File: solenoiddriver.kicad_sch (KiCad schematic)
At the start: 14 parts, among them Q501 WSP6946, Q502 WSP6946

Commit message: Assign footprints
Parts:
- D501, D502, D503, D504: footprint (none) -> Diode_SMD:D_SMA_Handsoldering
- R501, R502, R503, R504, R505, R506, R507, R508: footprint (none) -> Resistor_SMD:R_0805_2012Metric_Pad1.20x1.40mm_HandSolder
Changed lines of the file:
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@@
     (property "Reference" "R501" (id 0) (at 64.77 44.45 90))
     (property "Value" "150R" (id 1) (at 64.77 46.99 90))
-    (property "Footprint" "" (id 2) (at 64.77 48.768 90)
+    (property "Footprint" "Resistor_SMD:R_0805_2012Metric_Pad1.20x1.40mm_HandSolder" (id 2) (at 64.77 48.768 90)
       (effects (font (size 1.27 1.27)) hide)
     )
@@
     (property "Reference" "R502" (id 0) (at 64.77 76.2 90))
     (property "Value" "150R" (id 1) (at 64.77 78.74 90))
-    (property "Footprint" "" (id 2) (at 64.77 76.962 90)
+    (property "Footprint" "Resistor_SMD:R_0805_2012Metric_Pad1.20x1.40mm_HandSolder" (id 2) (at 64.77 76.962 90)
       (effects (font (size 1.27 1.27)) hide)
     )
@@
       (effects (font (size 1.27 1.27)) (justify left))
     )
-    (property "Footprint" "" (id 2) (at 69.342 52.07 90)
+    (property "Footprint" "Resistor_SMD:R_0805_2012Metric_Pad1.20x1.40mm_HandSolder" (id 2) (at 69.342 52.07 90)
       (effects (font (size 1.27 1.27)) hide)
     )
@@
       (effects (font (size 1.27 1.27)) (justify right))
     )
-    (property "Footprint" "" (id 2) (at 72.898 83.82 90)
+    (property "Footprint" "Resistor_SMD:R_0805_2012Metric_Pad1.20x1.40mm_HandSolder" (id 2) (at 72.898 83.82 90)
       (effects (font (size 1.27 1.27)) hide)
     )
@@
     (property "Reference" "R505" (id 0) (at 149.86 44.45 90))
     (property "Value" "150R" (id 1) (at 149.86 46.99 90))
-    (property "Footprint" "" (id 2) (at 149.86 48.768 90)
+    (property "Footprint" "Resistor_SMD:R_0805_2012Metric_Pad1.20x1.40mm_HandSolder" (id 2) (at 149.86 48.768 90)
       (effects (font (size 1.27 1.27)) hide)
     )
@@
     (property "Reference" "R506" (id 0) (at 149.86 76.2 90))
     (property "Value" "150R" (id 1) (at 149.86 78.74 90))
-    (property "Footprint" "" (id 2) (at 149.86 80.518 90)
+    (property "Footprint" "Resistor_SMD:R_0805_2012Metric_Pad1.20x1.40mm_HandSolder" (id 2) (at 149.86 80.518 90)
       (effects (font (size 1.27 1.27)) hide)
     )
@@
       (effects (font (size 1.27 1.27)) (justify left))
     )
-    (property "Footprint" "" (id 2) (at 154.432 52.07 90)
+    (property "Footprint" "Resistor_SMD:R_0805_2012Metric_Pad1.20x1.40mm_HandSolder" (id 2) (at 154.432 52.07 90)
       (effects (font (size 1.27 1.27)) hide)
     )
@@
       (effects (font (size 1.27 1.27)) (justify left))
     )
-    (property "Footprint" "" (id 2) (at 154.432 83.82 90)
+    (property "Footprint" "Resistor_SMD:R_0805_2012Metric_Pad1.20x1.40mm_HandSolder" (id 2) (at 154.432 83.82 90)
       (effects (font (size 1.27 1.27)) hide)
     )
@@
       (effects (font (size 1.27 1.27)) (justify left))
     )
-    (property "Footprint" "" (id 2) (at 100.33 33.02 0)
+    (property "Footprint" "Diode_SMD:D_SMA_Handsoldering" (id 2) (at 100.33 33.02 0)
       (effects (font (size 1.27 1.27)) hide)
     )
@@
       (effects (font (size 1.27 1.27)) (justify left))
     )
-    (property "Footprint" "" (id 2) (at 100.33 64.77 0)
+    (property "Footprint" "Diode_SMD:D_SMA_Handsoldering" (id 2) (at 100.33 64.77 0)
       (effects (font (size 1.27 1.27)) hide)
     )
@@
       (effects (font (size 1.27 1.27)) (justify left))
     )
-    (property "Footprint" "" (id 2) (at 185.42 33.02 0)
+    (property "Footprint" "Diode_SMD:D_SMA_Handsoldering" (id 2) (at 185.42 33.02 0)
       (effects (font (size 1.27 1.27)) hide)
     )
@@
       (effects (font (size 1.27 1.27)) (justify left))
     )
-    (property "Footprint" "" (id 2) (at 185.42 64.77 0)
+    (property "Footprint" "Diode_SMD:D_SMA_Handsoldering" (id 2) (at 185.42 64.77 0)
       (effects (font (size 1.27 1.27)) hide)
     )

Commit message: Start PCB
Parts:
- R501, R502, R503, R504, R505, R506, R507, R508: footprint Resistor_SMD:R_0805_2012Metric_Pad1.20x1.40mm_HandSolder -> Resistor_SMD:R_0603_1608Metric_Pad0.98x0.95mm_HandSolder
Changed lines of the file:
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@@
     (property "Reference" "R501" (id 0) (at 64.77 44.45 90))
     (property "Value" "150R" (id 1) (at 64.77 46.99 90))
-    (property "Footprint" "Resistor_SMD:R_0805_2012Metric_Pad1.20x1.40mm_HandSolder" (id 2) (at 64.77 48.768 90)
+    (property "Footprint" "Resistor_SMD:R_0603_1608Metric_Pad0.98x0.95mm_HandSolder" (id 2) (at 64.77 48.768 90)
       (effects (font (size 1.27 1.27)) hide)
     )
@@
     (property "Reference" "R502" (id 0) (at 64.77 76.2 90))
     (property "Value" "150R" (id 1) (at 64.77 78.74 90))
-    (property "Footprint" "Resistor_SMD:R_0805_2012Metric_Pad1.20x1.40mm_HandSolder" (id 2) (at 64.77 76.962 90)
+    (property "Footprint" "Resistor_SMD:R_0603_1608Metric_Pad0.98x0.95mm_HandSolder" (id 2) (at 64.77 76.962 90)
       (effects (font (size 1.27 1.27)) hide)
     )
@@
       (effects (font (size 1.27 1.27)) (justify left))
     )
-    (property "Footprint" "Resistor_SMD:R_0805_2012Metric_Pad1.20x1.40mm_HandSolder" (id 2) (at 69.342 52.07 90)
+    (property "Footprint" "Resistor_SMD:R_0603_1608Metric_Pad0.98x0.95mm_HandSolder" (id 2) (at 69.342 52.07 90)
       (effects (font (size 1.27 1.27)) hide)
     )
@@
       (effects (font (size 1.27 1.27)) (justify right))
     )
-    (property "Footprint" "Resistor_SMD:R_0805_2012Metric_Pad1.20x1.40mm_HandSolder" (id 2) (at 72.898 83.82 90)
+    (property "Footprint" "Resistor_SMD:R_0603_1608Metric_Pad0.98x0.95mm_HandSolder" (id 2) (at 72.898 83.82 90)
       (effects (font (size 1.27 1.27)) hide)
     )
@@
     (property "Reference" "R505" (id 0) (at 149.86 44.45 90))
     (property "Value" "150R" (id 1) (at 149.86 46.99 90))
-    (property "Footprint" "Resistor_SMD:R_0805_2012Metric_Pad1.20x1.40mm_HandSolder" (id 2) (at 149.86 48.768 90)
+    (property "Footprint" "Resistor_SMD:R_0603_1608Metric_Pad0.98x0.95mm_HandSolder" (id 2) (at 149.86 48.768 90)
       (effects (font (size 1.27 1.27)) hide)
     )
@@
     (property "Reference" "R506" (id 0) (at 149.86 76.2 90))
     (property "Value" "150R" (id 1) (at 149.86 78.74 90))
-    (property "Footprint" "Resistor_SMD:R_0805_2012Metric_Pad1.20x1.40mm_HandSolder" (id 2) (at 149.86 80.518 90)
+    (property "Footprint" "Resistor_SMD:R_0603_1608Metric_Pad0.98x0.95mm_HandSolder" (id 2) (at 149.86 80.518 90)
       (effects (font (size 1.27 1.27)) hide)
     )
@@
       (effects (font (size 1.27 1.27)) (justify left))
     )
-    (property "Footprint" "Resistor_SMD:R_0805_2012Metric_Pad1.20x1.40mm_HandSolder" (id 2) (at 154.432 52.07 90)
+    (property "Footprint" "Resistor_SMD:R_0603_1608Metric_Pad0.98x0.95mm_HandSolder" (id 2) (at 154.432 52.07 90)
       (effects (font (size 1.27 1.27)) hide)
     )
@@
       (effects (font (size 1.27 1.27)) (justify left))
     )
-    (property "Footprint" "Resistor_SMD:R_0805_2012Metric_Pad1.20x1.40mm_HandSolder" (id 2) (at 154.432 83.82 90)
+    (property "Footprint" "Resistor_SMD:R_0603_1608Metric_Pad0.98x0.95mm_HandSolder" (id 2) (at 154.432 83.82 90)
       (effects (font (size 1.27 1.27)) hide)
     )

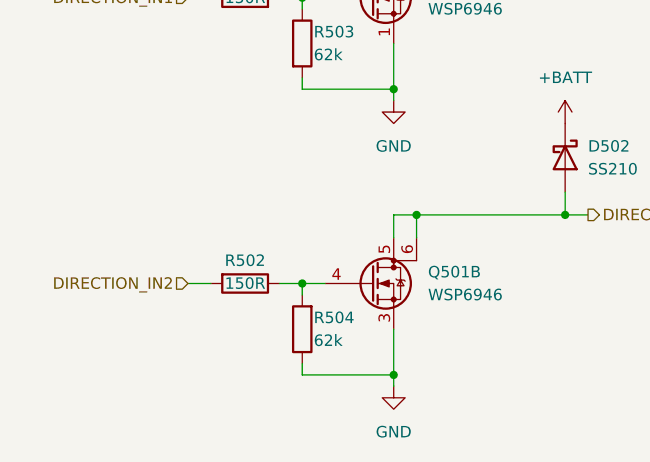
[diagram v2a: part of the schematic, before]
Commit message: Finish regulator layout
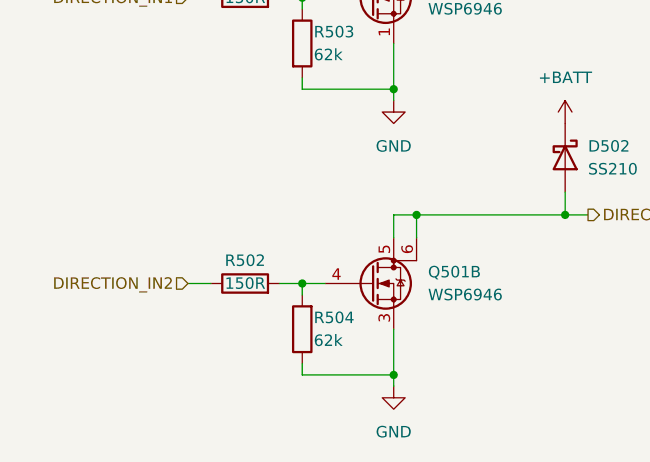
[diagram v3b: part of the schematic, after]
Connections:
- net DIRECTION_IN2: now also R502.1; no longer R502.2
- net at Q501.4 (G), R504.2: now also R502.2; no longer R502.1
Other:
- moved on the sheet: R502
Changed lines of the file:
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@@
     (pin "2")
   )
-  (symbol (lib_id "Device:R") (at 64.77 78.74 270) (unit 1)
+  (symbol (lib_id "Device:R") (at 64.77 78.74 90) (unit 1)
     (in_bom yes) (on_board yes)
     (property "Reference" "R502" (id 0) (at 64.77 76.2 90))
     (property "Value" "150R" (id 1) (at 64.77 78.74 90))
-    (property "Footprint" "Resistor_SMD:R_0603_1608Metric_Pad0.98x0.95mm_HandSolder" (id 2) (at 64.77 76.962 90)
+    (property "Footprint" "Resistor_SMD:R_0603_1608Metric_Pad0.98x0.95mm_HandSolder" (id 2) (at 64.77 80.518 90)
       (effects (font (size 1.27 1.27)) hide)
     )
